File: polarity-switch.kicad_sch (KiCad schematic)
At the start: 17 parts, among them U4 FDMQ8205A, U5 140356145400, U6 140356145400

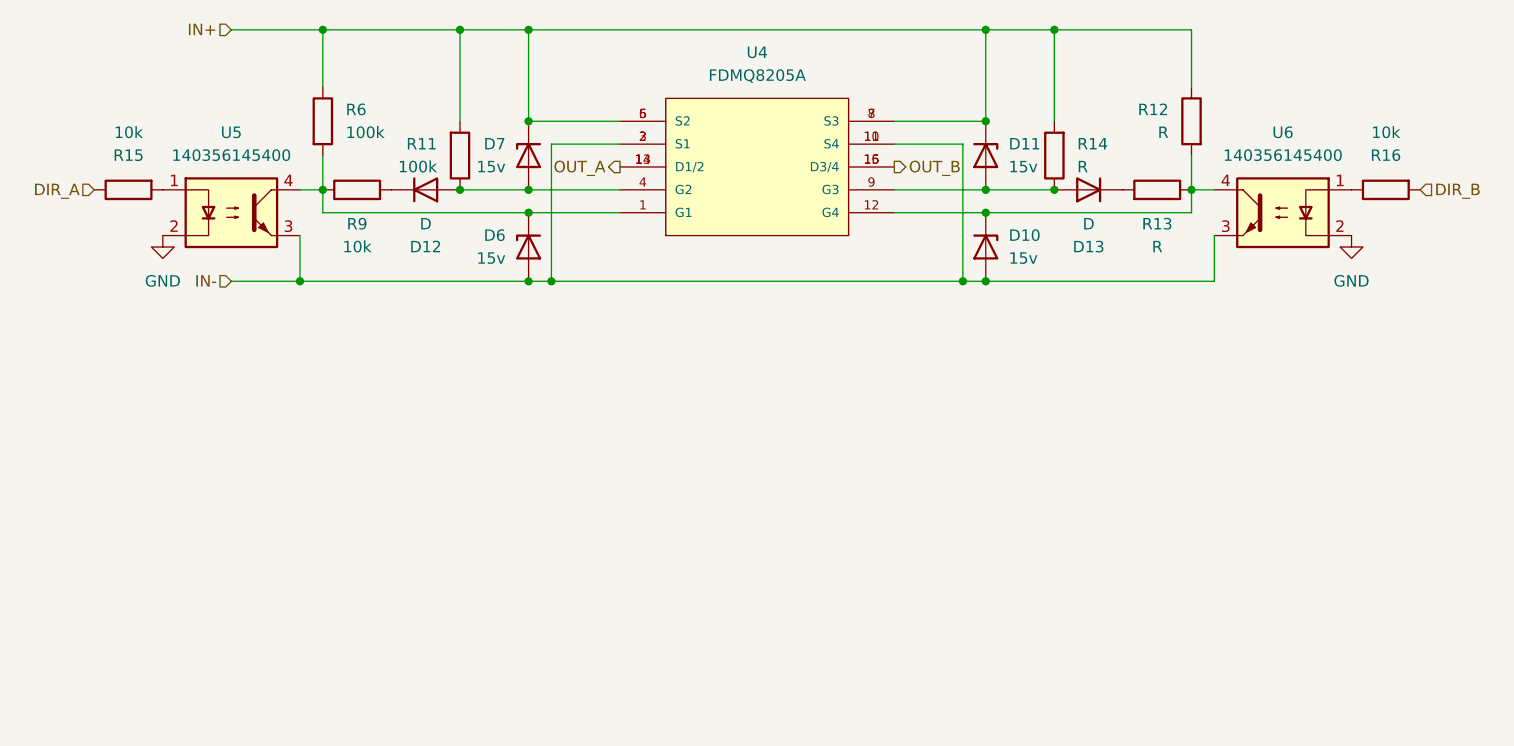
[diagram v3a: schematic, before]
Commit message: finished board
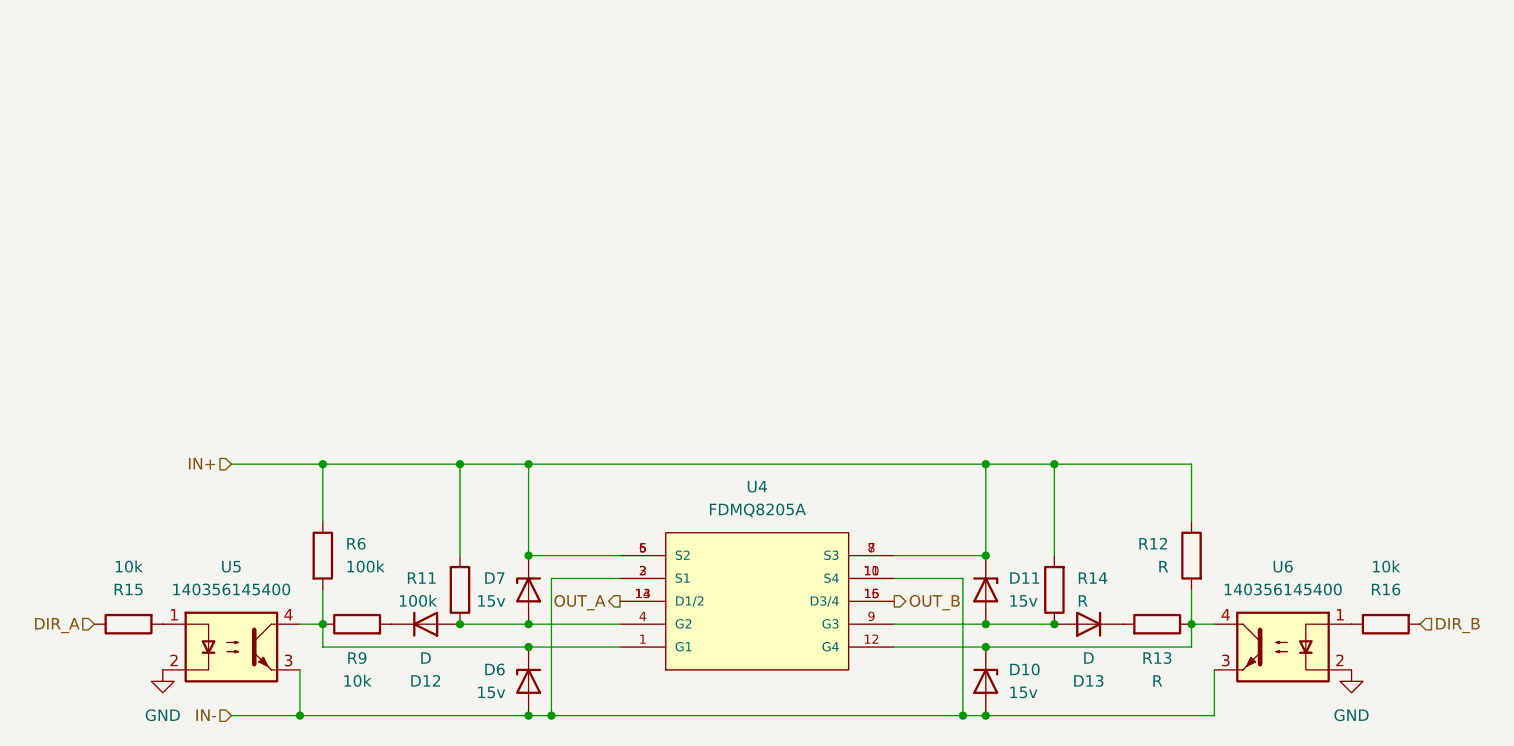
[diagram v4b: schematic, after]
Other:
- moved on the sheet: D10, D11, D12, D13, D6, D7, R11, R12, R13, R14, R15, R16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
